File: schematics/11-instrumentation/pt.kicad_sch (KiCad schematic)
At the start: 11 parts

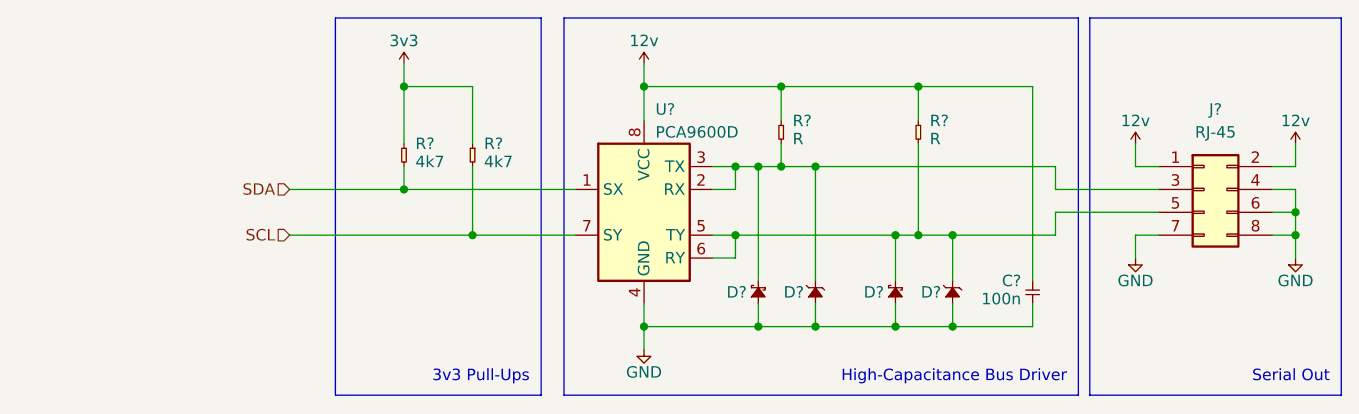
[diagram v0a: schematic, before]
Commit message: Added stuff
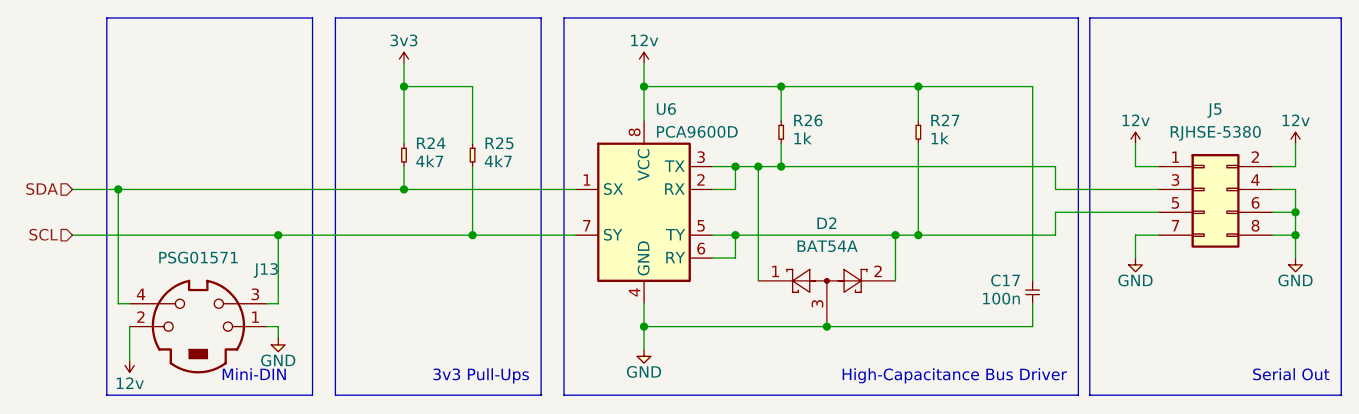
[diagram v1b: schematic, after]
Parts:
- removed D? (x2): Diode_Schottky, symbol royale:Diode_Schottky
- removed D? (x2): Diode_Zener, symbol royale:Diode_Zener
- added D2: BAT54A, Package_TO_SOT_SMD:SOT-23, symbol Diode:BAT54A
- added J13: PSG01571, royale:Mini-Din-Through-Hole, symbol Connector:Mini-DIN-4
- C17: renamed from C?; footprint (none) -> Capacitor_SMD:C_0805_2012Metric
- J5: renamed from J?; value RJ-45 -> RJHSE-5380; footprint (none) -> Connector_RJ:RJ45_Amphenol_RJHSE5380
- R24, R25: renamed from R?; footprint (none) -> Resistor_SMD:R_0805_2012Metric
- R26, R27: renamed from R?; value R -> 1k; footprint (none) -> Resistor_SMD:R_0805_2012Metric
- gave numbers to parts that had none: 1
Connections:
- net 3v3: now also J13.2
- net GND: now also D2.3, J13.1
- net SCL: now also J13.3
- net SDA: now also J13.4
- net at J5.3 (Pin_3), R26.2, U6.2 (RX)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: now also D2.1
- net at J5.5 (Pin_5), R27.2, U6.5 (TY)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: now also D2.2
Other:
- note added: "Mini-DIN"
